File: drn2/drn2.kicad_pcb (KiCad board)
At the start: 4 copper layers, 96.8 x 39.8 mm, 61 parts, among them J1 Conn_01x03_Socket, J2 Conn_01x04_Socket, J3 Conn_01x03_Socket, J37 Conn_01x03_Socket, J3_F2_BAT1 Conn_01x02_Pin, J4 Conn_01x03_Socket, J4_M0_MOT0 Conn_01x02_Pin, J4_M1_MOT1 Conn_01x02_Pin, J4_M2_MOT2 Conn_01x02_Pin, J4_M3_MOT3 Conn_01x02_Pin, J7 Conn_01x03_Socket, J9 Conn_01x04_Pin

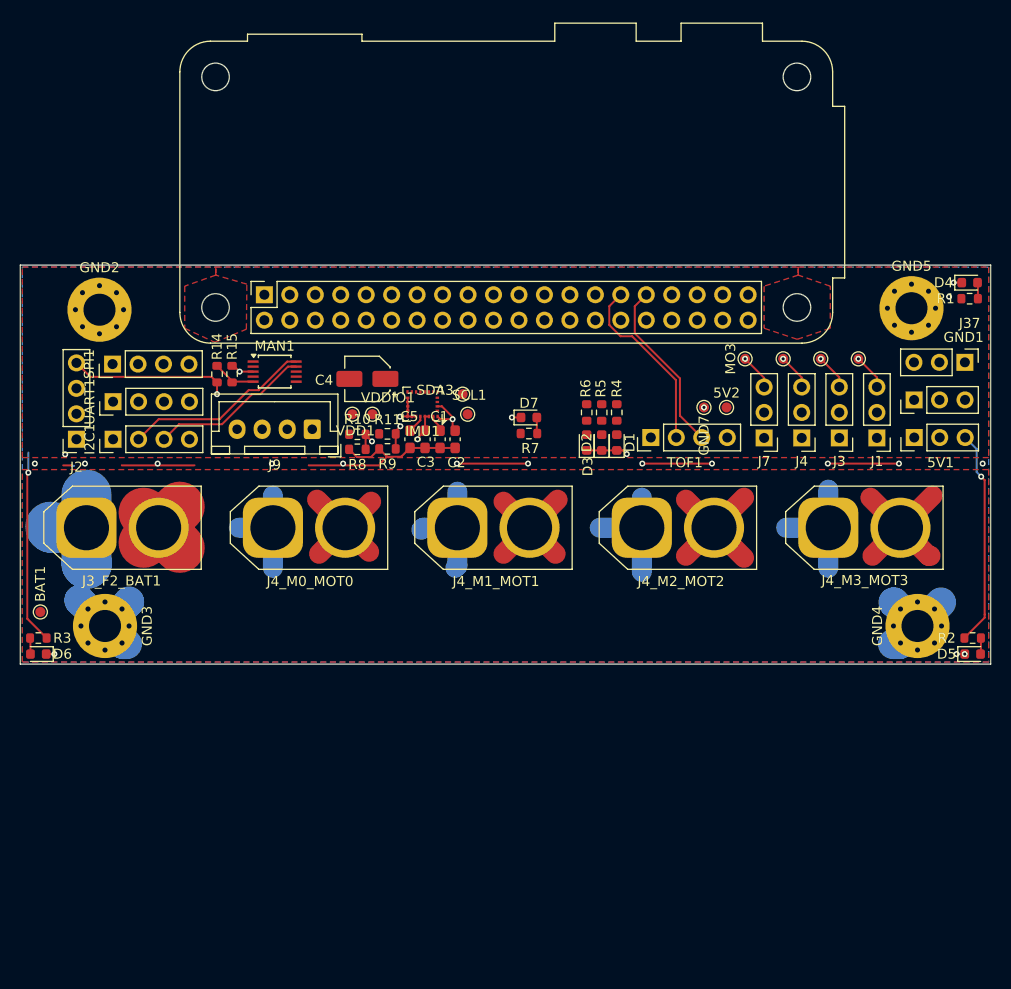
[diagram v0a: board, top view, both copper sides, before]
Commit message: v4 done, requires FP check
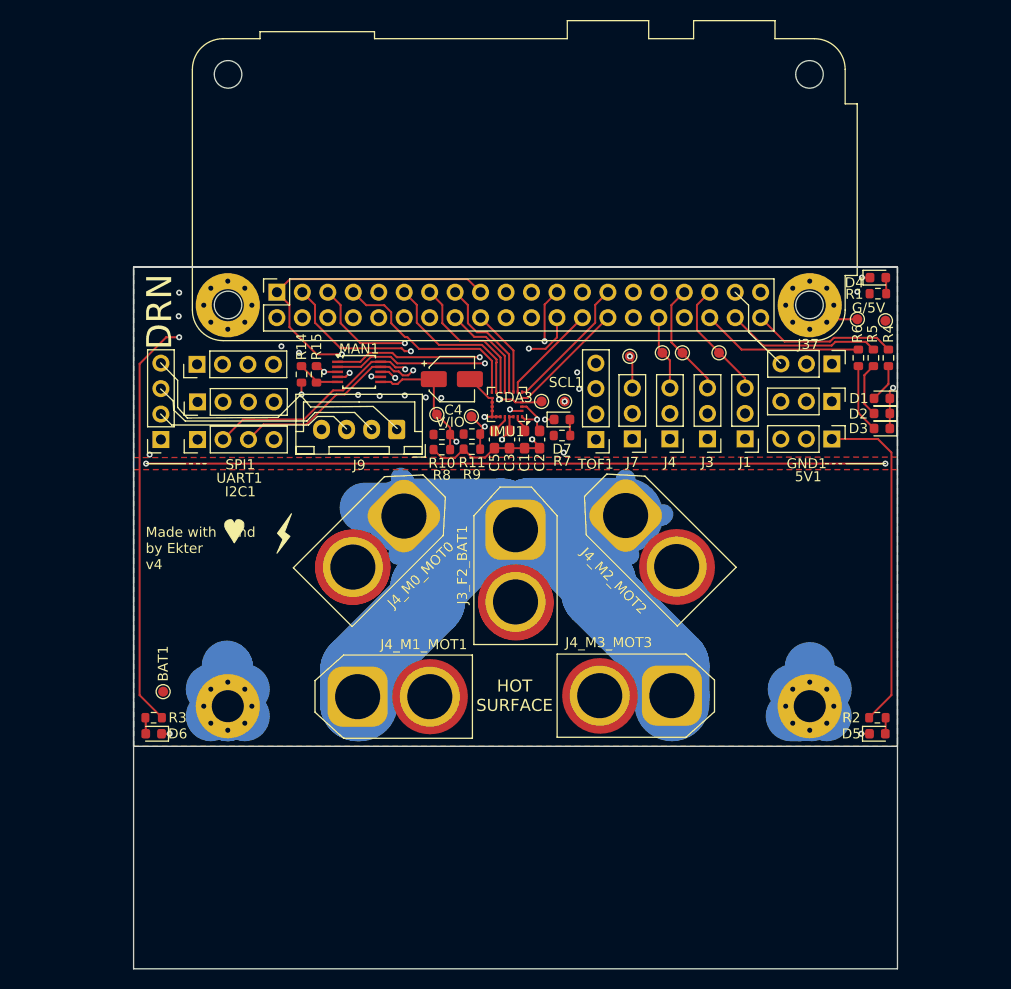
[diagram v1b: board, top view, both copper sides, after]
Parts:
- moved J3_F2_BAT1 42.8 mm to (112.2, 170.2), turned to -90 degrees
- moved D3 29.5 mm to (148.8, 160.1), turned to 180 degrees
- moved D2 28.1 mm to (148.8, 158.6), turned to 180 degrees
- moved R4 27.6 mm to (149.4, 153.1)
- moved R5 27.6 mm to (147.9, 153.1)
- moved R6 27.6 mm to (146.4, 153.1)
- moved D1 26.8 mm to (148.8, 157.1), turned to 180 degrees
- moved J4_M3_MOT3 22.9 mm to (127.8, 186.8), turned to 180 degrees
- moved J4_M1_MOT1 19.6 mm to (96.5, 186.8)
- moved 5V2 18.1 mm to (149.1, 149.3)
- moved GND7 17.7 mm to (146.3, 149.2)
- moved GND3 14.6 mm to (83.5, 187.8)
- moved BAT1 14.6 mm to (77.0, 186.3)
- moved D6 14.0 mm to (76.1, 190.6)
- moved R3 14.0 mm to (76.1, 188.9)
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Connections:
- RPI2 pad 15: Net-(IMU1-INT_M) -> Net-(IMU1-DRDY_M)
- RPI2 pad 16: Net-(IMU1-DRDY_M) -> Net-(IMU1-INT_M)
- SPI1 pad 2: Net-(RPI2-MOSI0/GPIO10) -> Net-(RPI2-MISO0/GPIO9)
- SPI1 pad 3: Net-(RPI2-MISO0/GPIO9) -> Net-(RPI2-MOSI0/GPIO10)
- TOF1 pad 2: Net-(RPI2-GCLK1/GPIO5) -> Net-(RPI2-GCLK2/GPIO6)
- TOF1 pad 3: Net-(RPI2-GCLK2/GPIO6) -> Net-(RPI2-GCLK1/GPIO5)
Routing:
- net /11.1: track 144.2 -> 0.90 mm
- net GND: track 286.2 -> 404.9 mm, vias 21 -> 11
- net Net-(RPI2-MISO0/GPIO9): track 0.00 -> 37.6 mm
- net /5V: track 41.0 -> 78.4 mm, vias 4 -> 15
- net Net-(I2C1-Pin_2): track 18.9 -> 55.9 mm, vias 0 -> 4
- net Net-(MAN1-AIN0): track 0.00 -> 35.3 mm, vias 0 -> 2
- net Net-(I2C1-Pin_3): track 16.2 -> 50.5 mm, vias 0 -> 3
- net Net-(RPI2-MOSI0/GPIO10): track 0.00 -> 31.8 mm
- net Net-(MAN1-ALERT/RDY): track 0.00 -> 27.7 mm, vias 0 -> 2
- net Net-(MAN1-ADDR): track 0.00 -> 25.2 mm, vias 0 -> 2
- net Net-(J7-Pin_3): track 3.60 -> 27.4 mm
- net Net-(IMU1-DEN_A/G): track 0.00 -> 20.4 mm
- net Net-(RPI2-GPIO15/RXD): track 0.00 -> 16.5 mm
- net Net-(RPI2-GPIO14/TXD): track 0.00 -> 16.5 mm
- net Net-(IMU1-INT2_A/G): track 0.00 -> 16.3 mm
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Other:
- board size 96.8 x 39.8 mm -> 76.2 x 70 mm
- board text added: "DRN"
- board text added: "G/5V"
- board text added: "HOT SURFACE"
- board text added: "Made with and by Ekter v4"
- board text added: "V/IO"
- board text added: "Warning! High current, PCB can get hot!"
- board text added: "github:ekter/drn"
